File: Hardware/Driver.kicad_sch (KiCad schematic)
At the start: 17 parts, among them J1 Motor, U1 MP6540

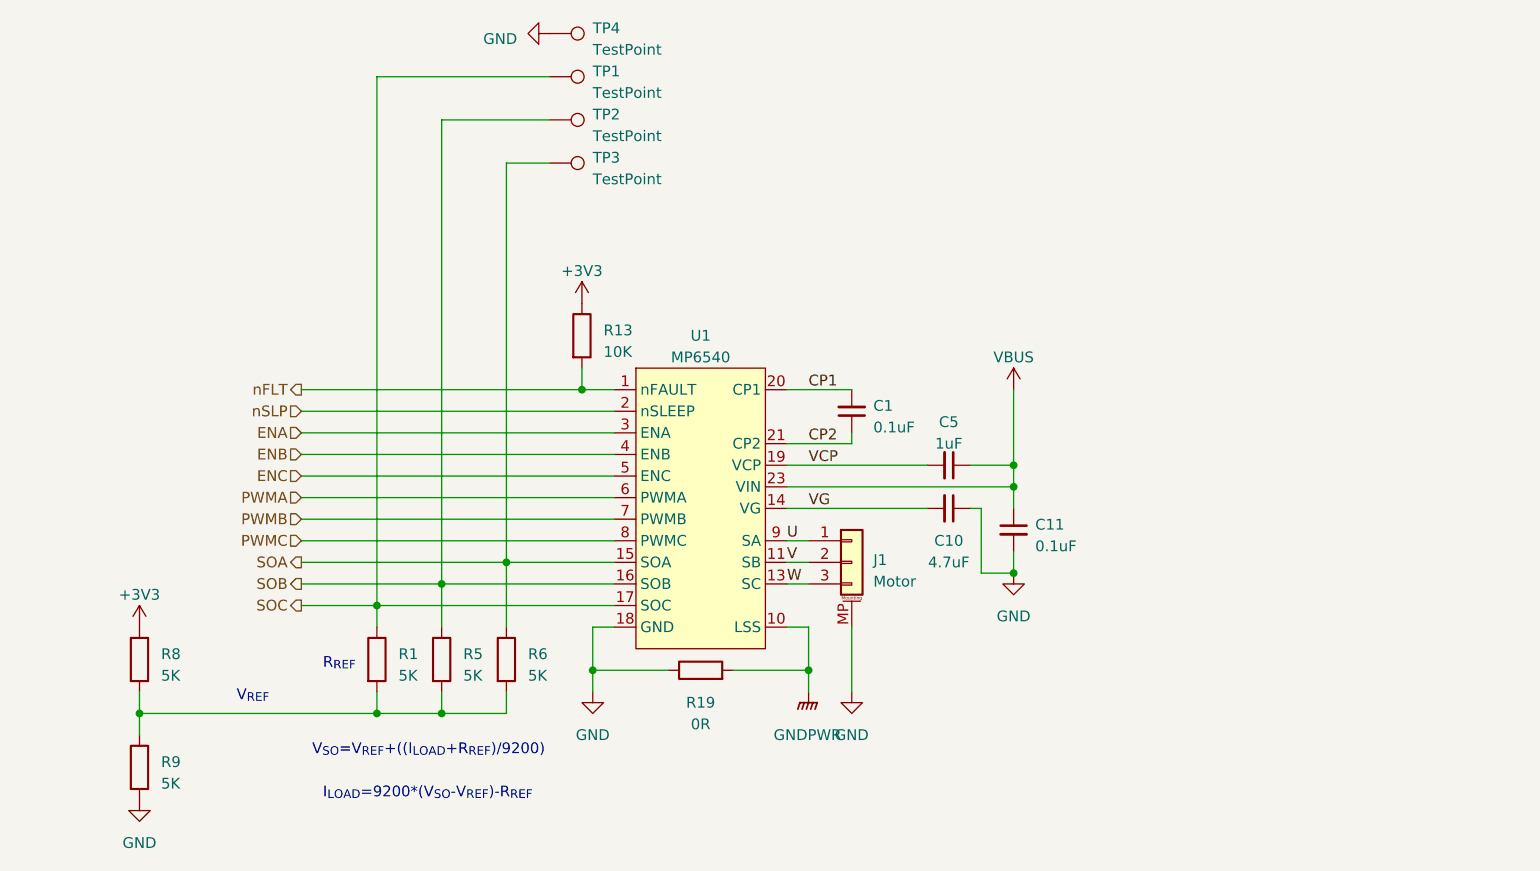
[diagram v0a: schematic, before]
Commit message: 调整第二版原理图
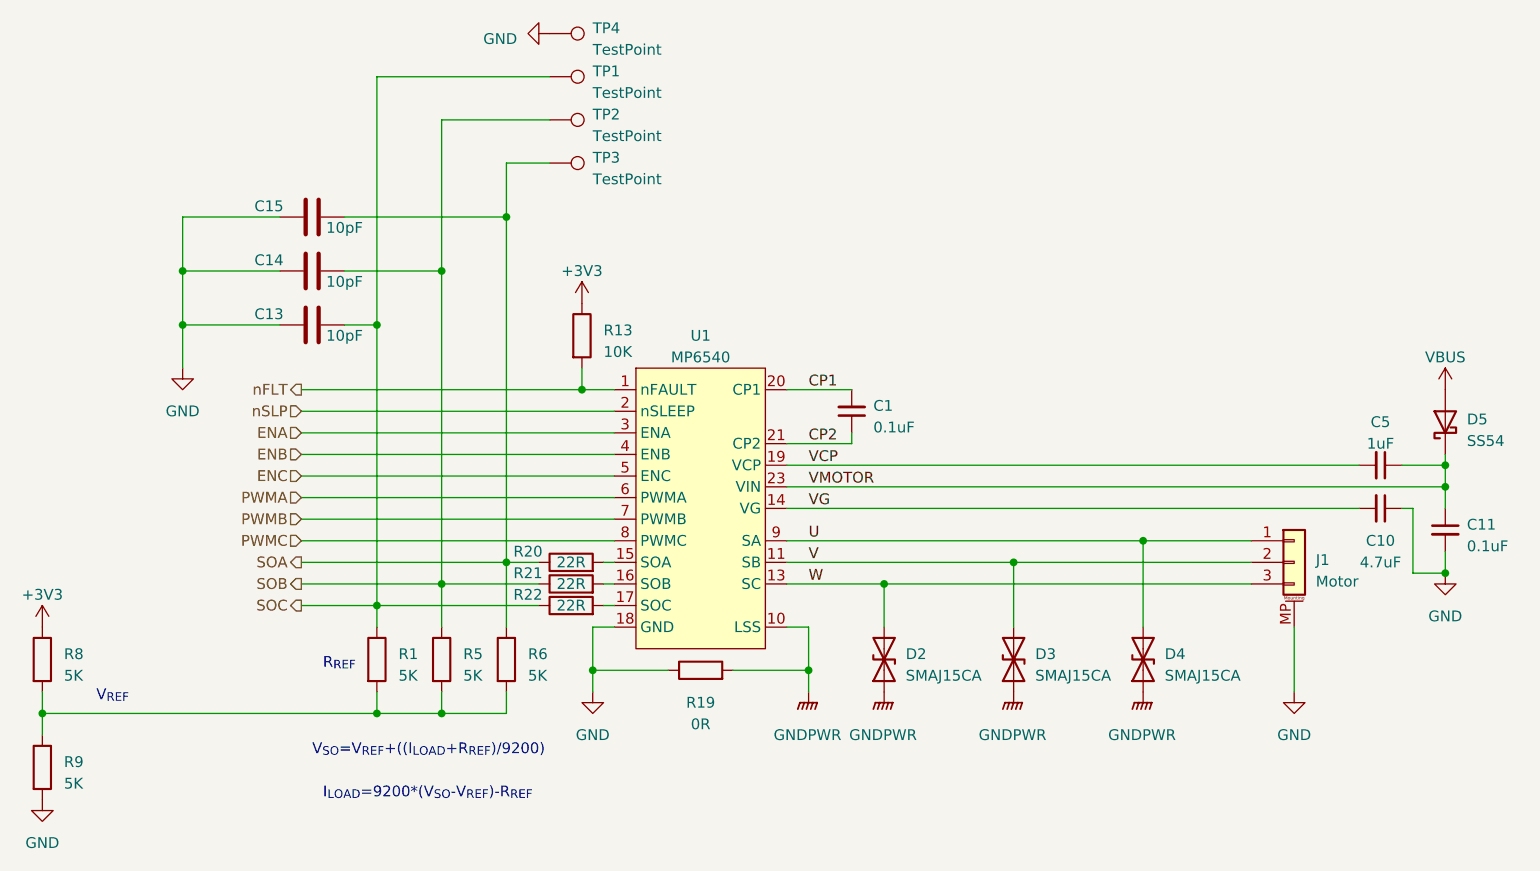
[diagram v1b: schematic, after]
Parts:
- added C13, C14, C15: 10pF, myDevice:0603_C, symbol Device:C
- added D2, D3, D4: SMAJ15CA, Diode_SMD:D_SMA, symbol Device:D_TVS
- added D5: SS54, Diode_SMD:D_SMB, symbol Device:D_Schottky
- added R20, R21, R22: 22R, myDevice:0603_R, symbol Device:R
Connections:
- net GND: now also C13.1, C14.1, C15.1
- net GNDPWR: now also D2.1 (A1), D3.1 (A1), D4.1 (A1)
- net SOA: now also C15.2, R20.1; no longer U1.15 (SOA)
- net SOB: now also C14.2, R21.1; no longer U1.16 (SOB)
- net SOC: now also C13.2, R22.1; no longer U1.17 (SOC)
- net U: now also D4.2 (A2)
- net V: now also D3.2 (A2)
- net VBUS: now also D5.2 (A); no longer C11.1, C5.1, U1.23 (VIN), U1.25 (VIN)
- net W: now also D2.2 (A2)
- new net: R21.2, U1.16 (SOB)
- new net: R22.2, U1.17 (SOC)
- new net: R20.2, U1.15 (SOA)
- new net VIN: C11.1, C5.1, D5.1 (K), U1.23 (VIN), U1.25 (VIN)
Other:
- moved on the sheet: C10, C11, C5, J1, R8, R9
